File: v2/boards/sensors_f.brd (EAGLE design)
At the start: 35.6 x 35.6 mm, 5 parts, among them U14 LINE_R, U15 LINE_L

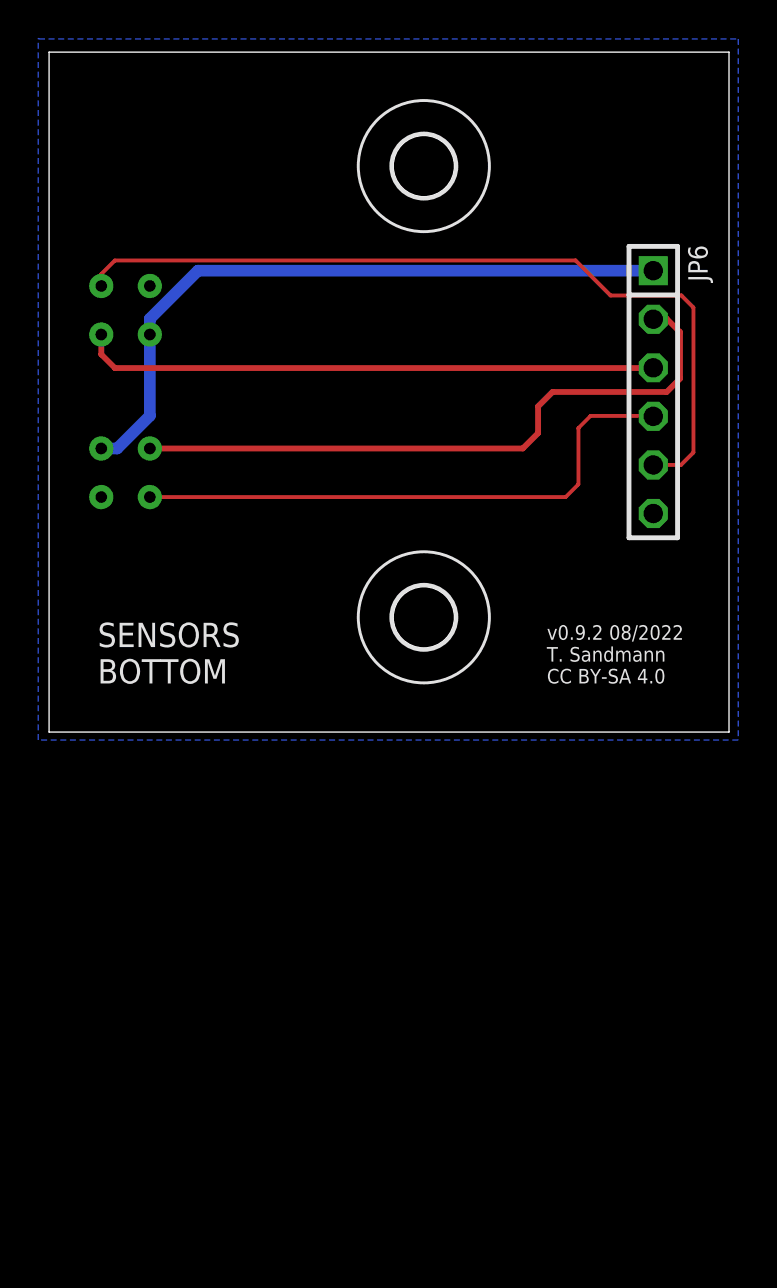
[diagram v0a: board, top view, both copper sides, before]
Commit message: schematics and board files for ct-Bot v2 prototype
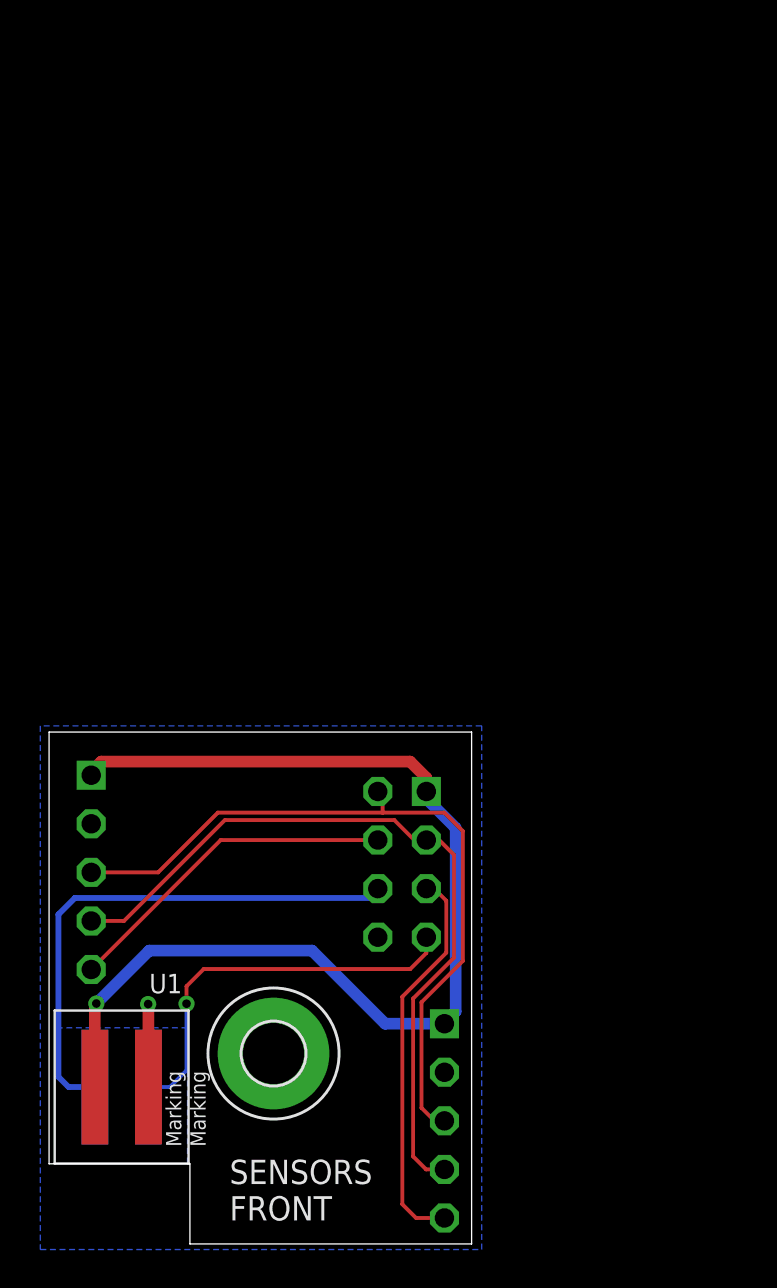
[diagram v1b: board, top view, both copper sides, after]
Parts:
- removed H2: MOUNT-HOLE3.2, myholes:3,2
- removed JP6: (no value), ct-bot:1X06
- removed U14: LINE_R, ct-bot:4
- removed U15: LINE_L, ct-bot:4
- added JP1: (no value), ct-bot:2X04
- added JP2: VL53L0X, ct-bot:1X05
- added JP3: VL6180X, ct-bot:1X05
- added U1: KANTE, ct-bot:EDGE
- H1: value MOUNT-HOLE3.2 -> MOUNT-PAD-ROUND3.2; device myholes:3,2 -> holes:3,2-PAD
- moved H1 47.1 mm to (11.7, -16.8)
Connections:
- removed net LINE_L: JP6.4, U15.C
- removed net LINE_R: JP6.5, U14.C
- removed net LOWSIDE_LINE_L: JP6.2, U15.K
- removed net LOWSIDE_LINE_R: JP6.3, U14.K
- new net D_SHDN: JP1.4, JP2.5
- new net KANTE: JP1.7, U1.COL
- new net LOWSIDE_KANTLED: JP1.6, U1.C
- new net SCL_5V: JP1.3, JP2.4, JP3.4
- new net SDA_5V: JP1.2, JP2.3, JP3.3
- new net T_SHDN: JP1.5, JP3.5
- net +5V: now also JP1.1, JP2.1, JP3.1, U1.A; no longer JP6.1, U14.A, U15.A
- net GND: now also JP1.8, JP2.2, JP3.2, U1.EMI; no longer JP6.6, U14.E, U15.E
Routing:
- net LINE_R: track 42.9 -> 0.00 mm
- net SCL_5V: track 0.00 -> 40.5 mm
- net SDA_5V: track 0.00 -> 39.2 mm
- net LOWSIDE_LINE_L: track 34.2 -> 0.00 mm
- net LOWSIDE_LINE_R: track 30.2 -> 0.00 mm
- net LINE_L: track 29.8 -> 0.00 mm
- net LOWSIDE_KANTLED: track 0.00 -> 28.0 mm
- net +5V: track 35.7 -> 57.4 mm, vias 0 -> 1
- net KANTE: track 0.00 -> 20.8 mm, vias 0 -> 1
- net T_SHDN: track 0.00 -> 20.6 mm
- net D_SHDN: track 0.00 -> 17.8 mm
- net GND: track 0.00 -> 4.34 mm, vias 0 -> 1
- added copper zone on layer 16, net N$1
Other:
- board size 35.6 x 35.6 mm -> 22.1 x 26.8 mm
- board text added: "SENSORS FRONT"
- board text added: "VL53L0X"
- board text added: "VL6180X"
- board text removed: "SENSORS BOTTOM"
